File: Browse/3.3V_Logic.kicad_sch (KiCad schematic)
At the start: 9 parts, among them IC6 TPS2121RUXT

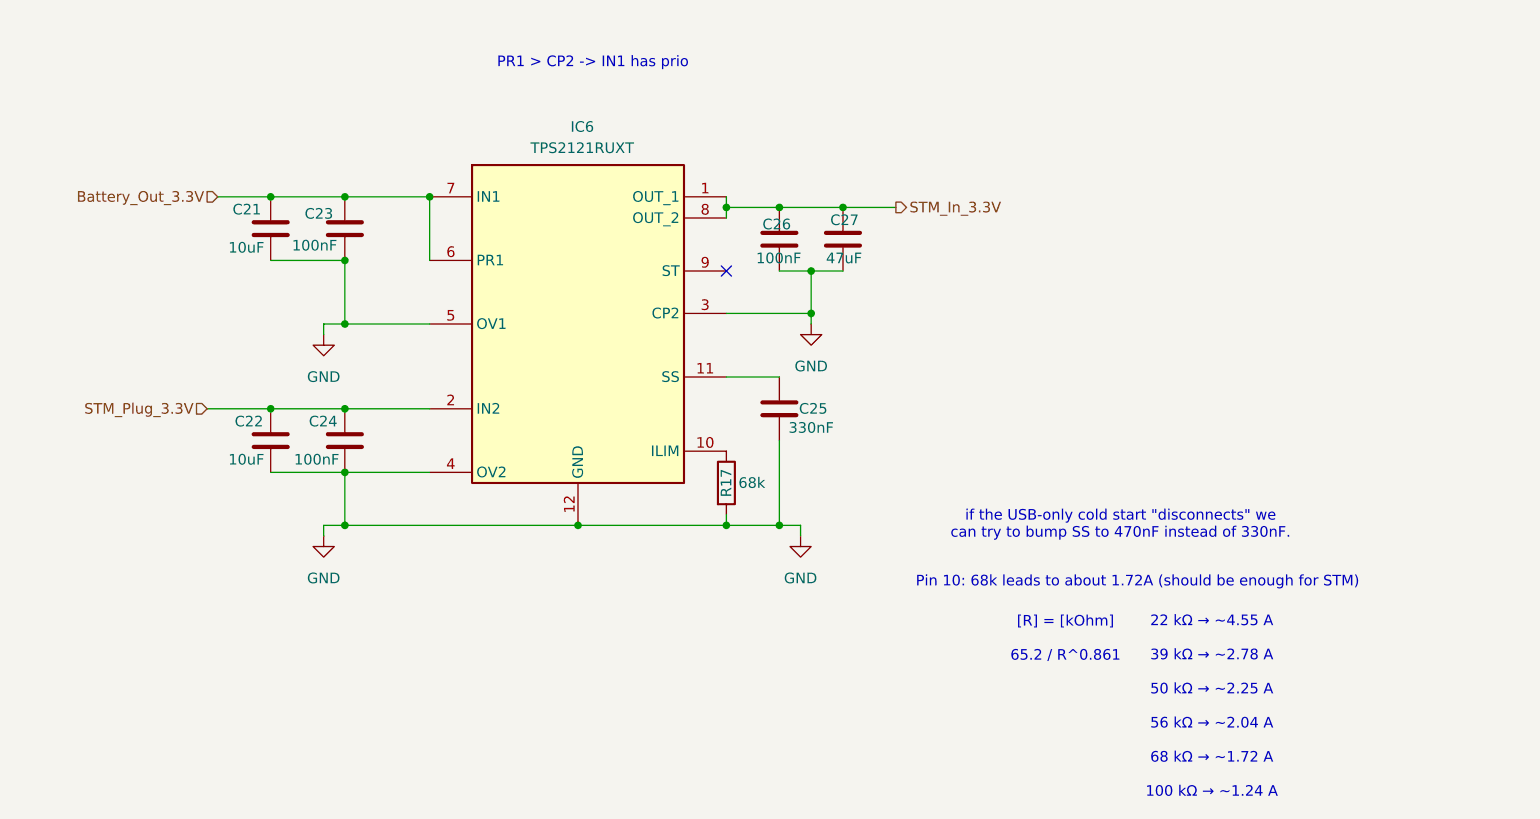
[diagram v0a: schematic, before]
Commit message: Deploying to gh-pages from @ Nautilus-UUV/nautilus-mainboard-PCB@5f5fdd9436d408a604bb268d740c0ac7ce1f5af5 🚀
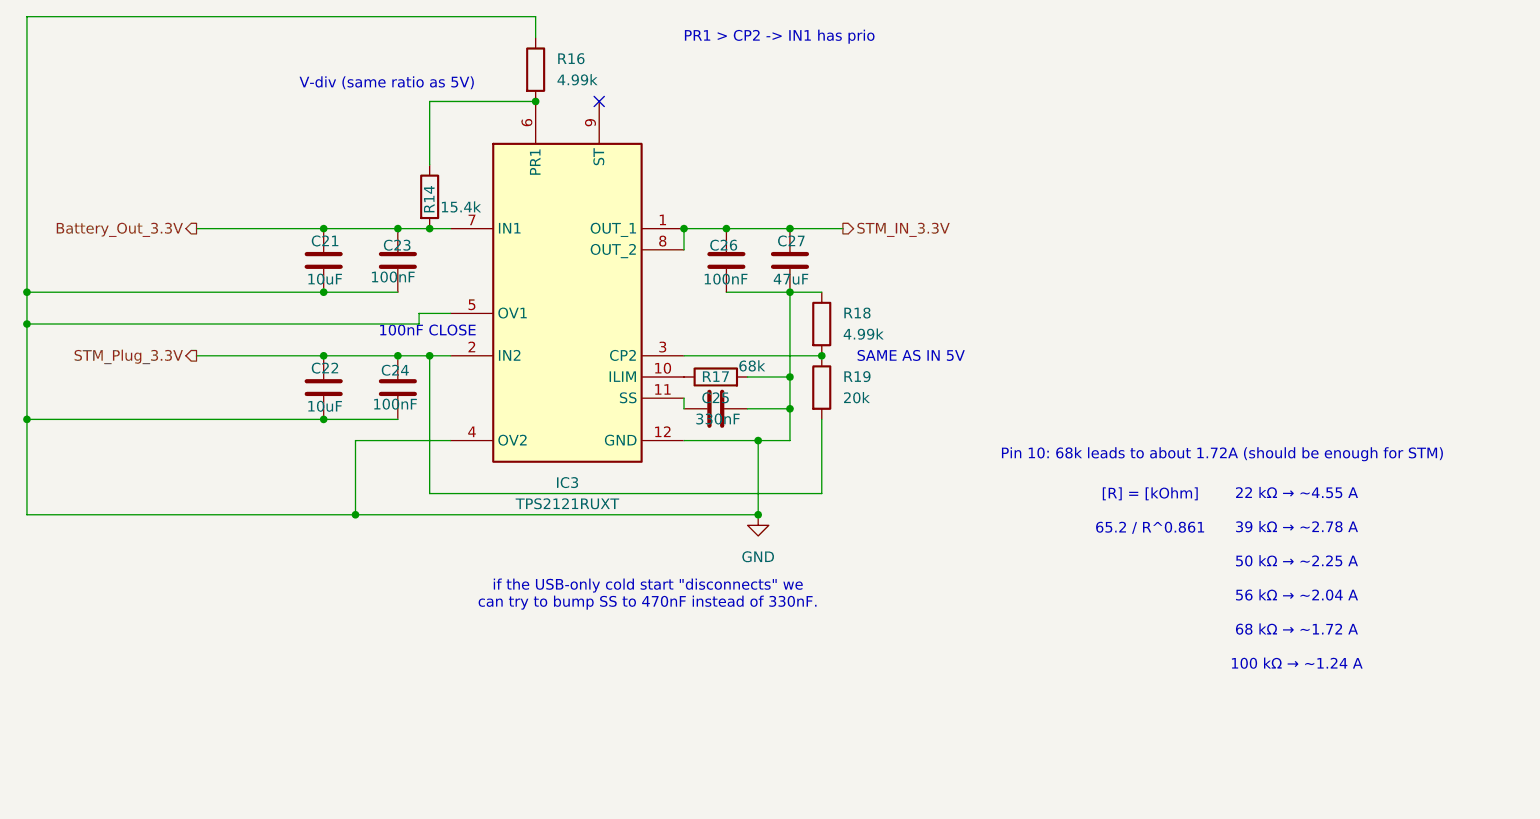
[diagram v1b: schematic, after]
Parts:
- removed IC6: TPS2121RUXT, dz_dio:TI_Switchover_TPS2121RUXT, symbol #dzdb:s_misc/TEXA-595-TPS2121RUXT
- added IC3: TPS2121RUXT, dz_dio:TI_Switchover_TPS2121RUXT, symbol #dzdb:s_misc/TEXA-595-TPS2121RUXT
- added R14: 15.4k, Resistor_SMD:R_0603_1608Metric, symbol #dzdb:g_res/R-15.4k-0603
- added R16, R18: 4.99k, Resistor_SMD:R_0603_1608Metric, symbol #dzdb:g_res/R-4.99k-0603
- added R19: 20k, Resistor_SMD:R_0603_1608Metric, symbol #dzdb:g_res/R-20k-0603
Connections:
- net Battery_Out_3.3V: now also IC3.7 (IN1), R14.2
- net GND: now also C25.2, IC3.12 (GND), IC3.4 (OV2), IC3.5 (OV1), R16.1, R18.1; no longer C25.1
- net STM_Plug_3.3V: now also IC3.2 (IN2), R19.2
- net at R17.1: now also IC3.10 (ILIM)
- net STM_In_3.3V renamed STM_IN_3.3V
- net STM_IN_3.3V: now also IC3.1 (OUT_1), IC3.8 (OUT_2)
- new net: C25.1, IC3.11 (SS)
- new net: IC3.3 (CP2), R18.2, R19.1
- new net: IC3.6 (PR1), R14.1, R16.2
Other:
- note added: "100nF CLOSE"
- note added: "SAME AS IN 5V"
- note added: "V-div (same ratio as 5V)"
- company: Davide -> (none)
- title: Nautilus_Mainboard -> (none)
- moved on the sheet: C21, C22, C23, C24, C25, C26, C27, R17
